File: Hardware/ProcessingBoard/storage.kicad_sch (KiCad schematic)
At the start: 13 parts, among them U401 W25Q32JVZP

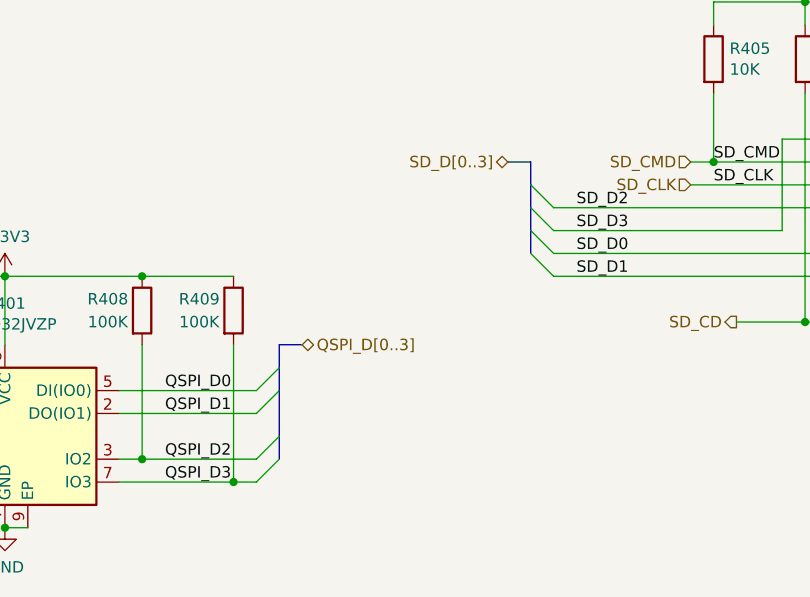
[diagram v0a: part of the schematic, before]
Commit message: pcb: switch to ad9978 wip
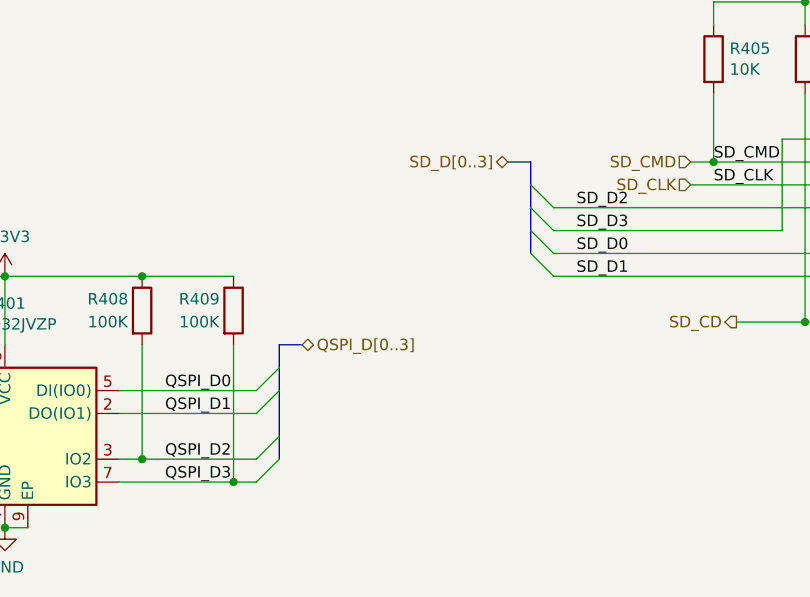
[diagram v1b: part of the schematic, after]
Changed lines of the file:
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@@
-(kicad_sch (version 20210126) (generator eeschema)
+(kicad_sch (version 20210621) (generator eeschema)
   (paper "A4")
   (title_block
@@
     (stroke (width 0) (type solid) (color 0 0 0 0))
   )
-  (bus (pts (xy 127 121.92) (xy 127 124.46))
+  (bus (pts (xy 127 121.92) (xy 127 134.62))
     (stroke (width 0) (type solid) (color 0 0 0 0))
   )
@@
     (stroke (width 0) (type solid) (color 0 0 0 0))
   )
-  (bus (pts (xy 127 124.46) (xy 127 127))
-    (stroke (width 0) (type solid) (color 0 0 0 0))
-  )
-  (bus (pts (xy 127 127) (xy 127 132.08))
-    (stroke (width 0) (type solid) (color 0 0 0 0))
-  )
-  (bus (pts (xy 127 132.08) (xy 127 134.62))
-    (stroke (width 0) (type solid) (color 0 0 0 0))
-  )
   (bus (pts (xy 154.94 101.6) (xy 152.4 101.6))
     (stroke (width 0) (type solid) (color 0 0 0 0))
   )
-  (bus (pts (xy 154.94 101.6) (xy 154.94 104.14))
-    (stroke (width 0) (type solid) (color 0 0 0 0))
-  )
-  (bus (pts (xy 154.94 104.14) (xy 154.94 106.68))
-    (stroke (width 0) (type solid) (color 0 0 0 0))
-  )
-  (bus (pts (xy 154.94 106.68) (xy 154.94 109.22))
-    (stroke (width 0) (type solid) (color 0 0 0 0))
-  )
-  (bus (pts (xy 154.94 109.22) (xy 154.94 111.76))
-    (stroke (width 0) (type solid) (color 0 0 0 0))
-  )
+  (bus (pts (xy 154.94 101.6) (xy 154.94 111.76))
+    (stroke (width 0) (type solid) (color 0 0 0 0))
+  )

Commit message: pcb: PB r0p2 and CB r0p3 freeze
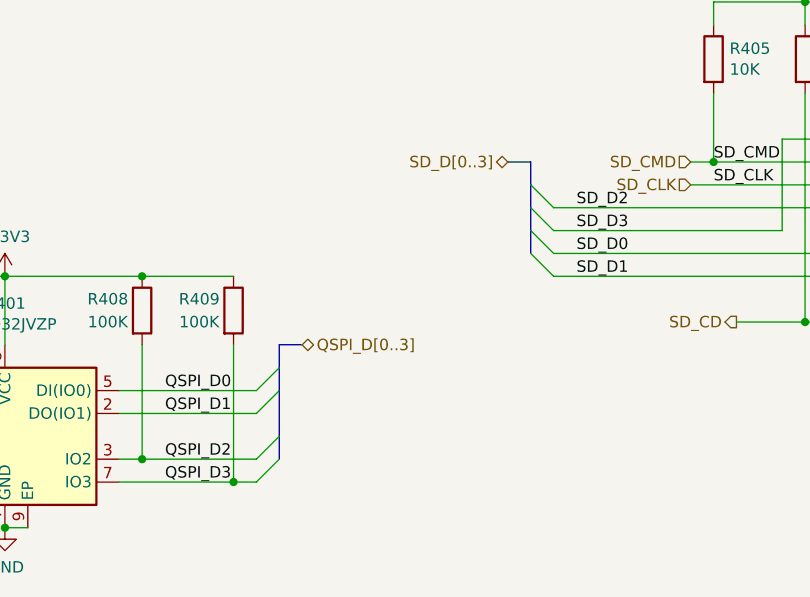
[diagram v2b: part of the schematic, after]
